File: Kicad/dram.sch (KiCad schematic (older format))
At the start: 13 parts, among them CN13 GVP_SIMM, CN14 GVP_SIMM, CN15 GVP_SIMM, CN16 GVP_SIMM, U45 74ABT16245, U46 74ABT16245, U47 74ABT16245, U48 74ABT16245, U49 SN74AS258, U50 SN74AS258

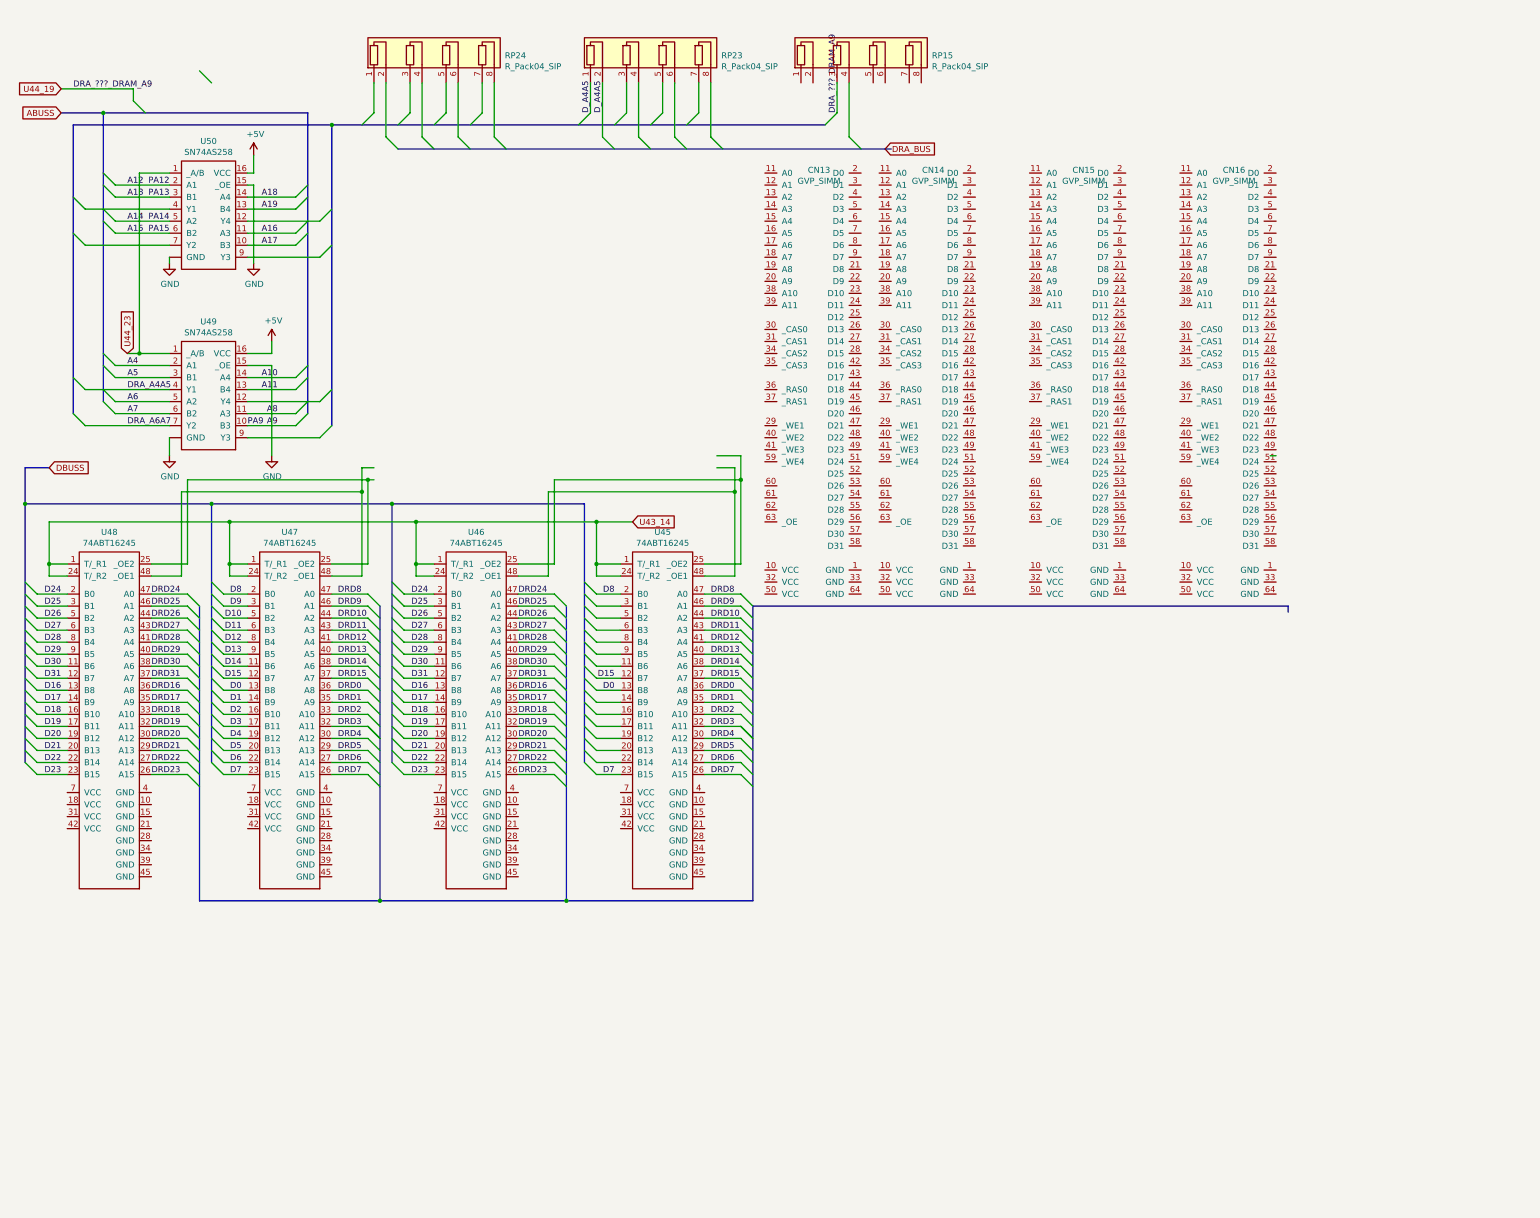
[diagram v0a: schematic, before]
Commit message: Some more work on dram
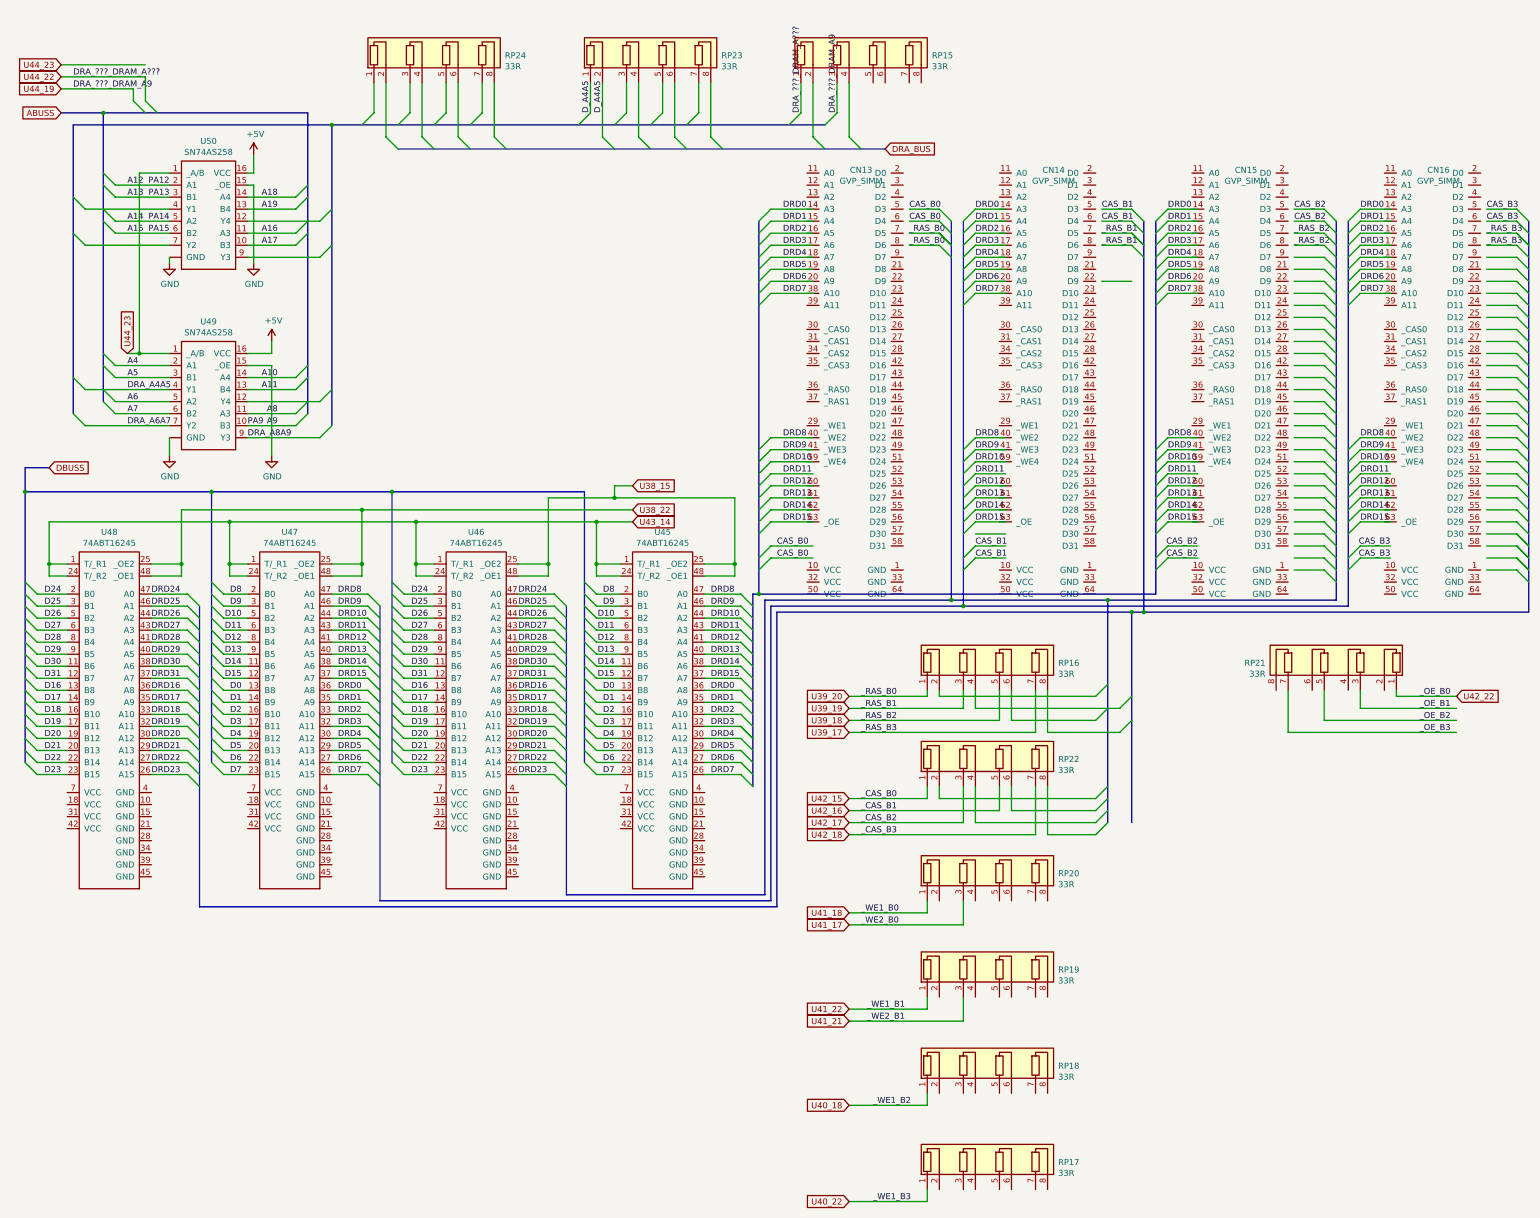
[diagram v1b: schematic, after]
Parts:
- added RP16, RP17, RP18, RP19, RP20, RP21, RP22: 33R, Resistor_THT:R_Array_SIP8, symbol Device:R_Pack04_SIP
- RP15, RP23, RP24: value R_Pack04_SIP -> 33R
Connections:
- net labels added: CAS_B0, CAS_B1, CAS_B2, CAS_B3, DRA_???_DRAM_A???, DRA_A8A9, U38_15, U38_22, U39_17, U39_18, U39_19, U39_20, U40_18, U40_22, U41_17, U41_18, U41_21, U41_22, U42_15, U42_16, U42_17, U42_18, U42_22, U44_22, _CAS_B0, _CAS_B1, _CAS_B2, _CAS_B3, _OE_B0, _OE_B1, _OE_B2, _OE_B3, _RAS_B0, _RAS_B1, _RAS_B2, _RAS_B3, _WE1_B0, _WE1_B1, _WE1_B2, _WE1_B3, _WE2_B0, _WE2_B1
- wire segments 234 -> 429
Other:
- moved on the sheet: CN13, CN14, CN15, CN16
